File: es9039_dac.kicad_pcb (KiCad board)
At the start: 4 copper layers, 65 x 68.6 mm, 92 parts, among them J1 Conn_02x07_Odd_Even, J2 XLR_L, J3 XLR_R, U1 ES9039Q2M, U2 TPS7A2033DBV, U3 LP5912-3.3DRV, U4 LP5912-3.3DRV, U5 TPS7A2033DBV, U6 OPA1612AxD, U7 OPA1612AxD, U8 OPA1612AxD, U9 OPA1612AxD

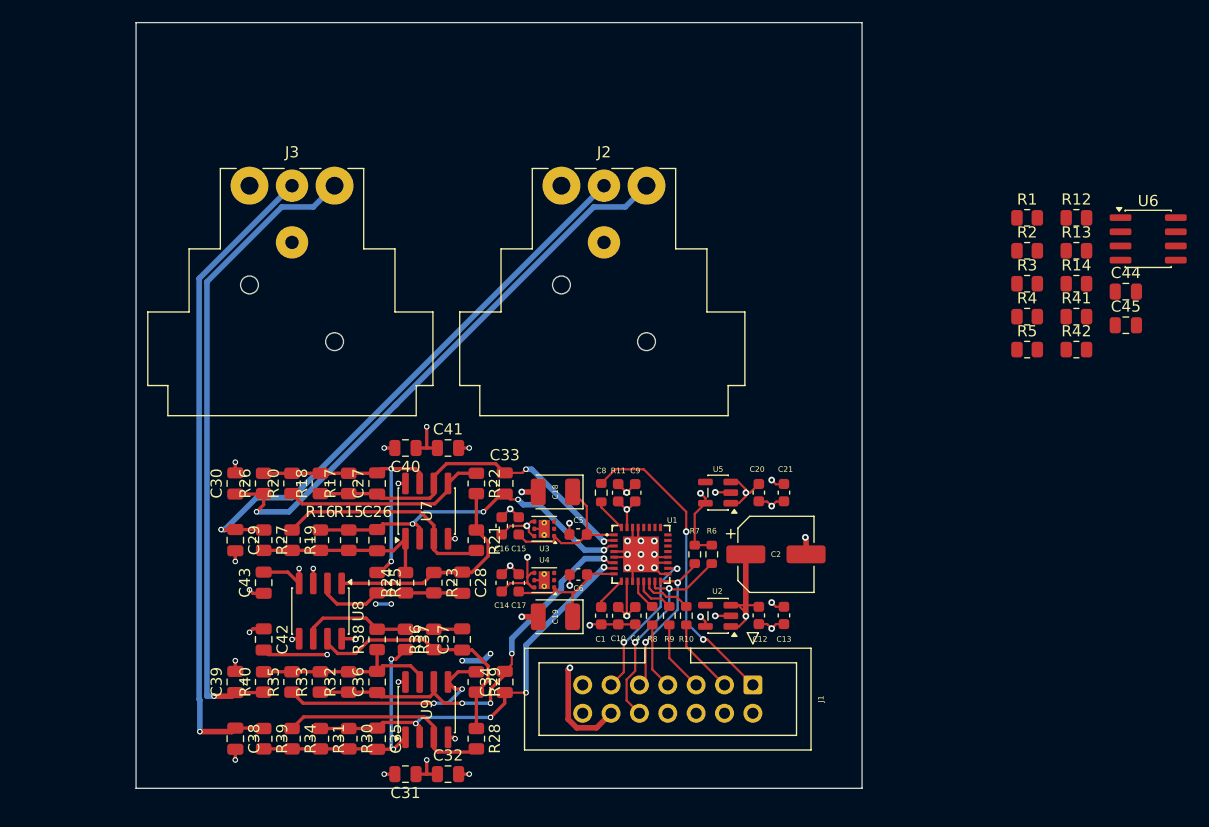
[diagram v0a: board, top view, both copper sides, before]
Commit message: add rca
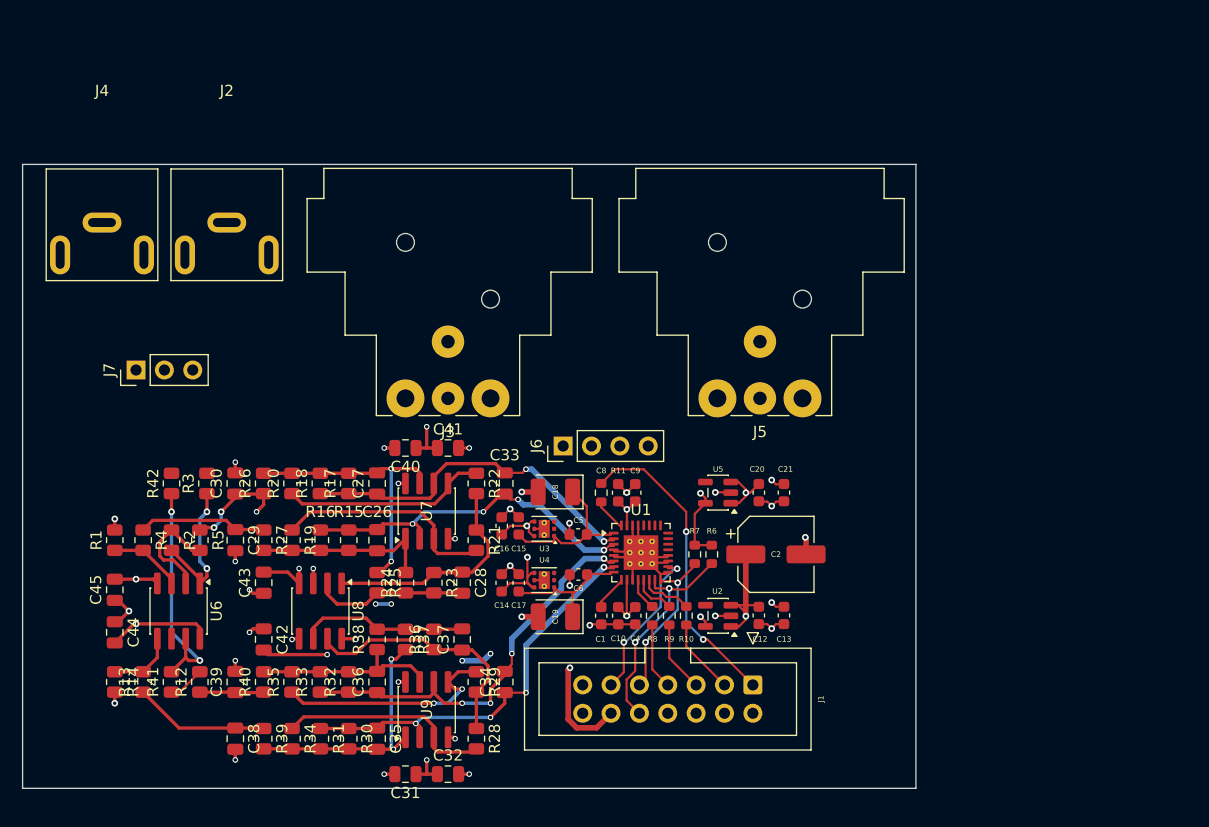
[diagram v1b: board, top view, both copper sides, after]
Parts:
- added J4: RCA_R, rca:RCA-105A, F.Cu at (172.2, 60.7)
- added J5: XLR_L, Connector_Audio:Jack_XLR_Neutrik_NC3MAH-0_Horizontal, F.Cu at (234.9, 81.3)
- added J6: BAL_OUT, Connector_PinHeader_2.54mm:PinHeader_1x04_P2.54mm_Vertical, F.Cu at (213.5, 85.5)
- added J7: UNBAL_OUT, Connector_PinHeader_2.54mm:PinHeader_1x03_P2.54mm_Vertical, F.Cu at (175.3, 78.7)
- J2: value XLR_L -> RCA_L; footprint Connector_Audio:Jack_XLR_Neutrik_NC3MAH-0_Horizontal -> rca:RCA-105A
- U1: footprint EasyEDA:QFN-32_L5.0-W5.0-P0.50-TL-EP3.2 -> Package_DFN_QFN:QFN-32-1EP_5x5mm_P0.5mm_EP3.1x3.1mm_ThermalVias
- moved C44 95.6 mm to (173.4, 102.2), turned to -90 degrees
- moved C45 93.6 mm to (173.4, 98.4), turned to 90 degrees
- moved R14 93.2 mm to (173.4, 106.7), turned to -90 degrees
- moved U6 93.0 mm to (179.1, 100.3), turned to -90 degrees
- moved R13 92.1 mm to (175.9, 106.7), turned to 90 degrees
- moved R12 88.8 mm to (181.0, 106.7), turned to 90 degrees
- moved R41 87.4 mm to (178.4, 106.7), turned to 90 degrees
- moved R1 86.7 mm to (173.4, 94.0), turned to 90 degrees
- moved R42 81.9 mm to (178.4, 88.9), turned to 90 degrees
- moved R4 81.7 mm to (175.9, 94.0), turned to -90 degrees
- moved R2 80.9 mm to (178.4, 94.0), turned to -90 degrees
- moved R5 76.0 mm to (181.0, 94.0), turned to -90 degrees
- moved R3 75.6 mm to (181.6, 88.9), turned to 90 degrees
- moved J2 30.0 mm to (183.4, 60.7)
- moved J3 28.8 mm to (207.0, 81.3), turned to 180 degrees
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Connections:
- J2 pad 1: GNDA -> UNBAL_OUT_L
- J2 pad 2: OUT_Lb -> GNDA
- J2 pad 3: OUT_L -> (no net)
- J3 pad G: (no net) -> GNDA
- U6 pad 4: unconnected-(U6C-V--Pad4) -> -12V
- U6 pad 8: unconnected-(U6C-V+-Pad8) -> +12V
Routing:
- net OUT_Rb: track 57.3 -> 5.75 mm, vias 1 -> 0
- net OUT_R: track 58.2 -> 12.1 mm, vias 1 -> 0
- net OUT_Lb: track 51.8 -> 9.60 mm, vias 1 -> 3
- net OUT_L: track 50.9 -> 11.5 mm, vias 1 -> 0
- net +12V: track 69.0 -> 96.7 mm, vias 8 -> 9
- net Net-(R41-Pad2): track 0.00 -> 20.9 mm, vias 0 -> 2
- net -12V: track 68.6 -> 87.5 mm, vias 7 -> 8
- net Net-(R2-Pad2): track 0.00 -> 12.8 mm, vias 0 -> 2
- net Net-(U6A--): track 0.00 -> 9.98 mm
- net Net-(U6A-+): track 0.00 -> 6.55 mm
- net Net-(U6B-+): track 0.00 -> 6.03 mm
- net GNDA: track 64.0 -> 69.3 mm, vias 32 -> 26
- net Net-(U6B--): track 0.00 -> 3.30 mm
- added copper zone on In1.Cu, net GNDA
- removed copper zone on In1.Cu, net (none)
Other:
- board size 65 x 68.6 mm -> 80 x 55.9 mm
